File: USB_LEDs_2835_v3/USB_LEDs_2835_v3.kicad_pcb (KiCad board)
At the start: 2 copper layers, 159 x 133.3 mm, 389 parts, among them J12 Screw_Terminal_01x03, J13 Barrel_Jack_Switch, U1 MT9284, U16 MT9284, U17 JL8022W-L, U18 74LVC1G04, U19 MT9284, U2 JL8022W-L, U20 JL8022W-L, U21 74LVC1G04, U22 MT9284, U23 JL8022W-L, U24 74LVC1G04, U25 MT9284, U26 JL8022W-L, U27 74LVC1G04, U3 74LVC1G04

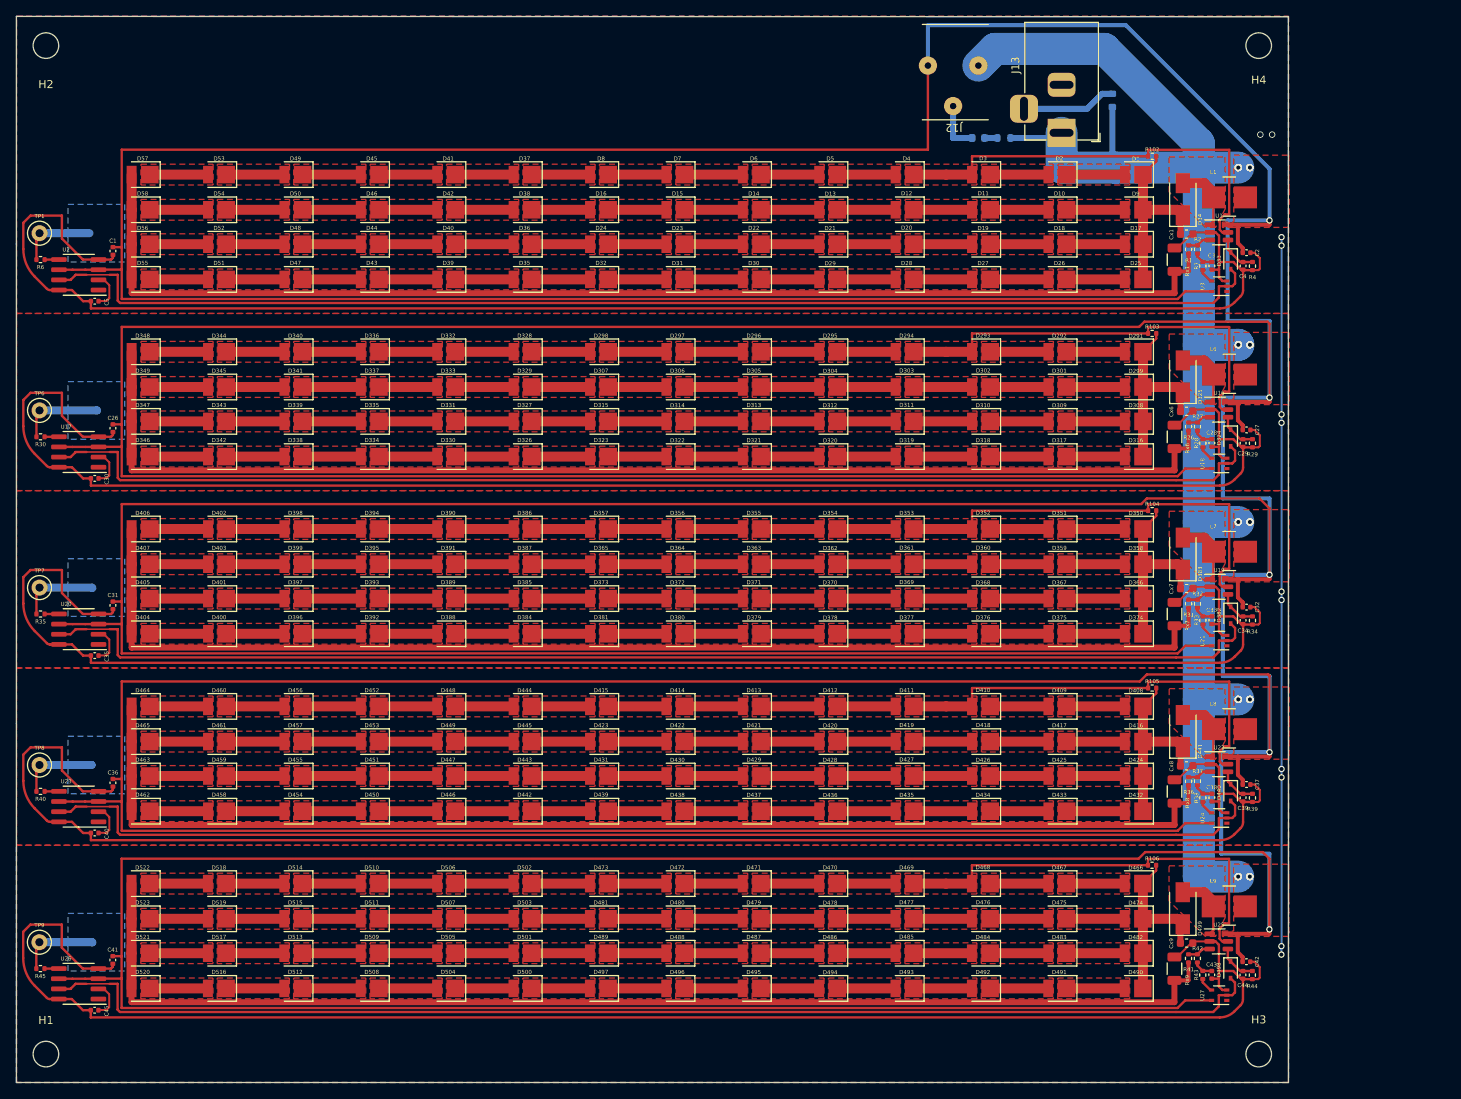
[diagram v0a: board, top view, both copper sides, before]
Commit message: Add files via upload
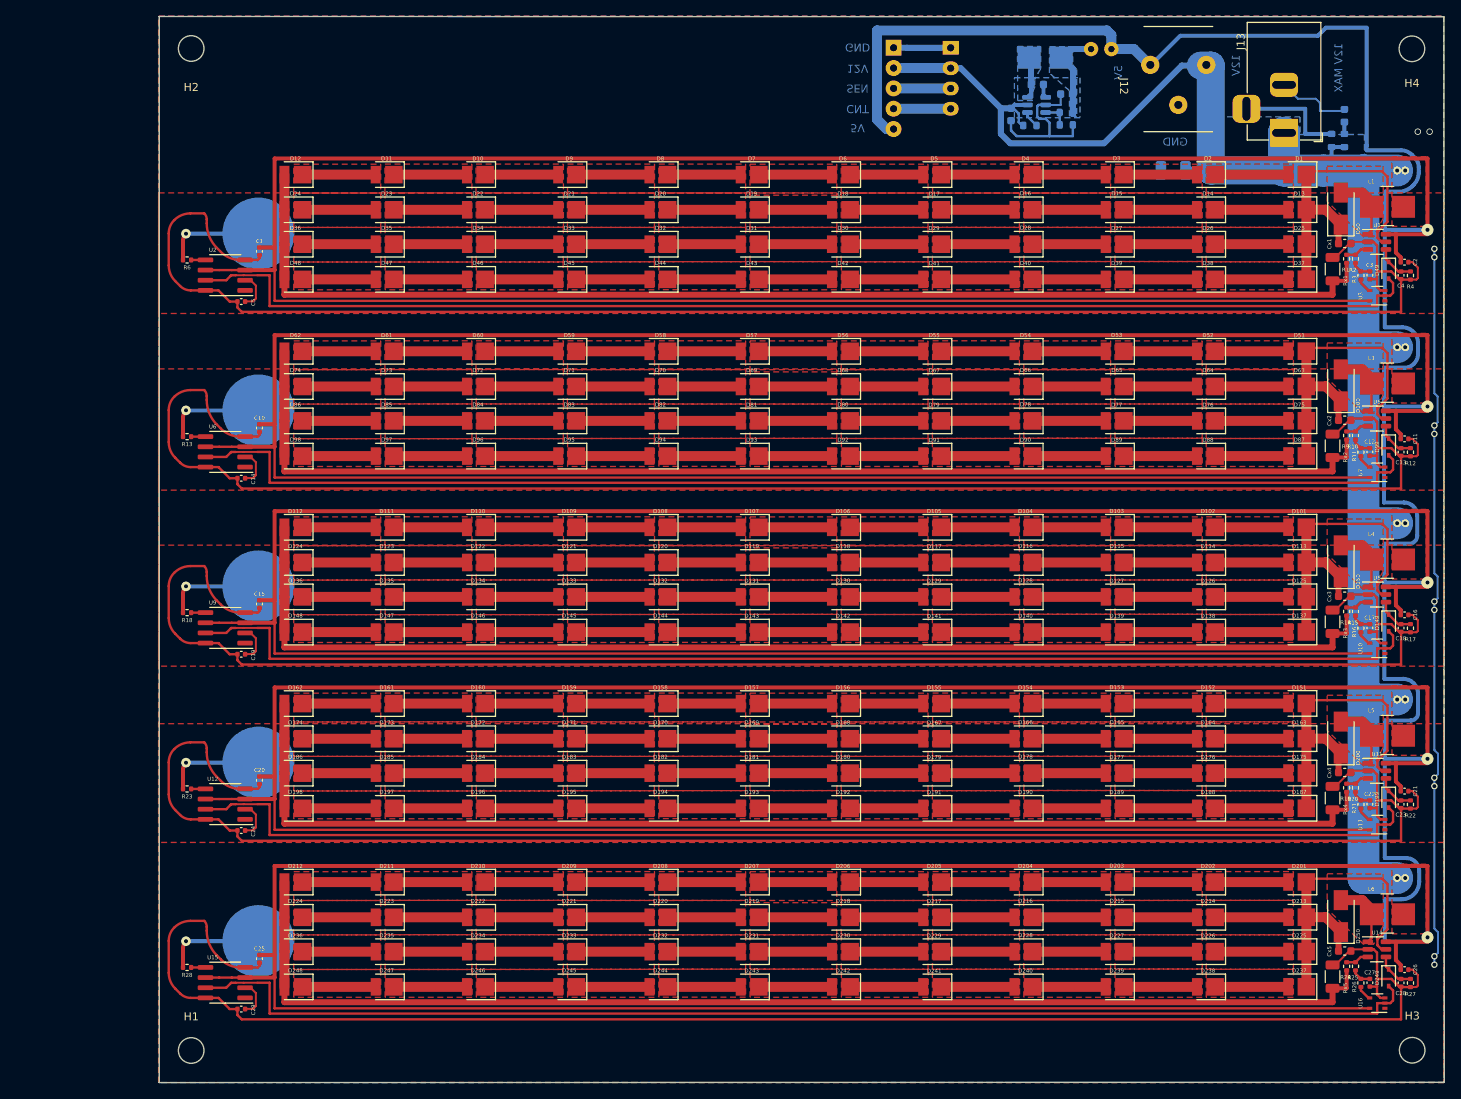
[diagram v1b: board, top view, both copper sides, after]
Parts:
- removed C30, C35, C40, C45: 10n, Capacitor_SMD:C_0402_1005Metric
- removed C31, C32, C33, C36, C37, C38, C41, C42, C43: 1u, Capacitor_SMD:C_0402_1005Metric
- removed C34, C39, C44: 1n, Capacitor_SMD:C_0402_1005Metric
- removed Cx6, Cx7, Cx8, Cx9: 1u, Capacitor_SMD:C_0603_1608Metric
- removed D291, D292, D293, D294, D295, D296, D297, D298, D299, D301, D302, D303, D304, D305, D306, D307, D308, D309, D310, D311, D312, D313, D314, D315, D316, D317, D318, D319, D320, D321, D322, D323, D326, D327, D328, D329, D330, D331, D332, D333, D334, D335, D336, D337, D338, D339, D340, D341, D342, D343, D344, D345, D346, D347, D348, D349, D350, D351, D352, D353, D354, D355, D356, D357, D358, D359, D360, D361, D362, D363, D364, D365, D366, D367, D368, D369, D370, D371, D372, D373, D374, D375, D376, D377, D378, D379, D380, D381, D384, D385, D386, D387, D388, D389, D390, D391, D392, D393, D394, D395, D396, D397, D398, D399, D400, D401, D402, D403, D404, D405, D406, D407, D408, D409, D410, D411, D412, D413, D414, D415, D416, D417, D418, D419, D420, D421, D422, D423, D424, D425, D426, D427, D428, D429, D430, D431, D432, D433, D434, D435, D436, D437, D438, D439, D442, D443, D444, D445, D446, D447, D448, D449, D450, D451, D452, D453, D454, D455, D456, D457, D458, D459, D460, D461, D462, D463, D464, D465, D466, D467, D468, D469, D470, D471, D472, D473, D474, D475, D476, D477, D478, D479, D480, D481, D482, D483, D484, D485, D486, D487, D488, D489, D490, D491, D492, D493, D494, D495, D496, D497, D500, D501, D502, D503, D504, D505, D506, D507, D508, D509, D510, D511, D512, D513, D514, D515, D516, D517, D518, D519, D520, D521, D522, D523: 660nm, LED_SMD:LED_2835
- removed D324, D382, D440, D498: 1N4148WS, Diode_SMD:D_SOD-323
- removed D325, D383, D441, D499: SS14, Diode_SMD:D_SMA
- removed L7, L8, L9: L_Ferrite_Small, Inductor_SMD:L_0530_custom
- removed R102, R103, R104, R105, R106: 500k, Resistor_SMD:R_0402_1005Metric
- removed R29, R34, R39, R44: 100k, Resistor_SMD:R_0402_1005Metric
- removed R30, R31, R35, R36, R40, R41, R45: 5k, Resistor_SMD:R_0402_1005Metric
- removed R32, R33, R37, R38, R42, R43: 10k, Resistor_SMD:R_0402_1005Metric
- removed Rx6, Rx7, Rx8, Rx9: 100m, Resistor_SMD:R_1206_3216Metric
- removed TP1, TP6, TP7, TP8, TP9: TestPoint, TestPoint:TestPoint_Loop_D2.50mm_Drill1.0mm
- removed U17, U20, U23, U26: JL8022W-L, Package_SO:SOIC-8_3.9x4.9mm_P1.27mm
- removed U18, U21, U24, U27: 74LVC1G04, Package_TO_SOT_SMD:SOT-353_SC-70-5
- removed U19, U22, U25: MT9284, Package_TO_SOT_SMD:SOT-23-6
- added ?: , , F.Cu at (82.5, 139.3)
- added ?: , , F.Cu at (82.5, 95.0)
- added ?: , , F.Cu at (82.5, 73.0)
- added ?: , , F.Cu at (82.5, 117.0)
- added C10: 1u, Capacitor_SMD:C_0402_1005Metric, F.Cu at (82.6, 75.2)
- added C11: 1u, Capacitor_SMD:C_0402_1005Metric, F.Cu at (225.7, 76.5)
- added C12: 1u, Capacitor_SMD:C_0402_1005Metric, F.Cu at (221.4, 78.2)
- added C13: 1n, Capacitor_SMD:C_0402_1005Metric, F.Cu at (225.3, 78.2)
- added C14: 10n, Capacitor_SMD:C_0402_1005Metric, F.Cu at (80.3, 81.5)
- added C15: 1u, Capacitor_SMD:C_0402_1005Metric, F.Cu at (82.6, 97.2)
- added C16: 1u, Capacitor_SMD:C_0402_1005Metric, F.Cu at (225.7, 98.5)
- added C17: 1u, Capacitor_SMD:C_0402_1005Metric, F.Cu at (221.4, 100.2)
- added C18: 1n, Capacitor_SMD:C_0402_1005Metric, F.Cu at (225.3, 100.2)
- added C19: 10n, Capacitor_SMD:C_0402_1005Metric, F.Cu at (80.3, 103.5)
- added C20: 1u, Capacitor_SMD:C_0402_1005Metric, F.Cu at (82.6, 119.2)
- added C21: 1u, Capacitor_SMD:C_0402_1005Metric, F.Cu at (225.7, 120.6)
- added C22: 1u, Capacitor_SMD:C_0402_1005Metric, F.Cu at (221.4, 122.2)
- added C23: 1n, Capacitor_SMD:C_0402_1005Metric, F.Cu at (225.3, 122.2)
- added C24: 10n, Capacitor_SMD:C_0402_1005Metric, F.Cu at (80.3, 125.5)
- added C25: 1u, Capacitor_SMD:C_0402_1005Metric, F.Cu at (82.6, 141.5)
- added C6: 22u, Capacitor_SMD:C_0603_1608Metric, B.Cu at (176.5, 36.0)
- added C7: 200n, Capacitor_SMD:C_0603_1608Metric, B.Cu at (179.8, 32.2)
- added C8: 22u, Capacitor_SMD:C_0603_1608Metric, B.Cu at (183.5, 33.5)
- added C9: 100u/16V, Capacitor_Tantalum_SMD:CP_EIA-3528-21_Kemet-B, B.Cu at (196.8, 43.0)
- added Cx2: 1u, Capacitor_SMD:C_0603_1608Metric, F.Cu at (218.2, 74.2)
- added Cx3: 1u, Capacitor_SMD:C_0603_1608Metric, F.Cu at (218.2, 96.2)
- added Cx4: 1u, Capacitor_SMD:C_0603_1608Metric, F.Cu at (218.2, 118.2)
- added Cx5: 1u, Capacitor_SMD:C_0603_1608Metric, F.Cu at (218.2, 140.6)
- added D100: SS14, Diode_SMD:D_SMA, F.Cu at (217.8, 69.9)
- added D101: 660nm, LED_SMD:LED_2835, F.Cu at (212.6, 87.6)
- added D102: 660nm, LED_SMD:LED_2835, F.Cu at (201.1, 87.6)
- added D103: 660nm, LED_SMD:LED_2835, F.Cu at (189.7, 87.6)
- added D104: 660nm, LED_SMD:LED_2835, F.Cu at (178.3, 87.6)
- added D105: 660nm, LED_SMD:LED_2835, F.Cu at (166.9, 87.6)
- added D106: 660nm, LED_SMD:LED_2835, F.Cu at (155.5, 87.6)
- added D107: 660nm, LED_SMD:LED_2835, F.Cu at (144.1, 87.6)
- added D108: 660nm, LED_SMD:LED_2835, F.Cu at (132.7, 87.6)
- added D109: 660nm, LED_SMD:LED_2835, F.Cu at (121.3, 87.6)
- added D110: 660nm, LED_SMD:LED_2835, F.Cu at (109.9, 87.6)
- added D111: 660nm, LED_SMD:LED_2835, F.Cu at (98.5, 87.6)
- added D112: 660nm, LED_SMD:LED_2835, F.Cu at (87.1, 87.6)
- added D113: 660nm, LED_SMD:LED_2835, F.Cu at (212.6, 92.0)
- added D114: 660nm, LED_SMD:LED_2835, F.Cu at (201.1, 92.0)
- added D115: 660nm, LED_SMD:LED_2835, F.Cu at (189.7, 92.0)
- added D116: 660nm, LED_SMD:LED_2835, F.Cu at (178.3, 92.0)
- added D117: 660nm, LED_SMD:LED_2835, F.Cu at (166.9, 92.0)
- added D118: 660nm, LED_SMD:LED_2835, F.Cu at (155.5, 92.0)
- added D119: 660nm, LED_SMD:LED_2835, F.Cu at (144.1, 92.0)
- added D120: 660nm, LED_SMD:LED_2835, F.Cu at (132.7, 92.0)
- added D121: 660nm, LED_SMD:LED_2835, F.Cu at (121.3, 92.0)
- added D122: 660nm, LED_SMD:LED_2835, F.Cu at (109.9, 92.0)
- added D123: 660nm, LED_SMD:LED_2835, F.Cu at (98.5, 92.0)
- added D124: 660nm, LED_SMD:LED_2835, F.Cu at (87.1, 92.0)
- added D125: 660nm, LED_SMD:LED_2835, F.Cu at (212.6, 96.3)
- added D126: 660nm, LED_SMD:LED_2835, F.Cu at (201.1, 96.3)
- added D127: 660nm, LED_SMD:LED_2835, F.Cu at (189.7, 96.3)
- added D128: 660nm, LED_SMD:LED_2835, F.Cu at (178.3, 96.3)
- added D129: 660nm, LED_SMD:LED_2835, F.Cu at (166.9, 96.3)
- added D130: 660nm, LED_SMD:LED_2835, F.Cu at (155.5, 96.3)
- added D131: 660nm, LED_SMD:LED_2835, F.Cu at (144.1, 96.3)
- added D132: 660nm, LED_SMD:LED_2835, F.Cu at (132.7, 96.3)
- added D133: 660nm, LED_SMD:LED_2835, F.Cu at (121.3, 96.3)
- added D134: 660nm, LED_SMD:LED_2835, F.Cu at (109.9, 96.3)
- added D135: 660nm, LED_SMD:LED_2835, F.Cu at (98.5, 96.3)
- added D136: 660nm, LED_SMD:LED_2835, F.Cu at (87.1, 96.3)
- added D137: 660nm, LED_SMD:LED_2835, F.Cu at (212.6, 100.7)
- added D138: 660nm, LED_SMD:LED_2835, F.Cu at (201.1, 100.7)
- added D139: 660nm, LED_SMD:LED_2835, F.Cu at (189.7, 100.7)
- added D140: 660nm, LED_SMD:LED_2835, F.Cu at (178.3, 100.7)
- added D141: 660nm, LED_SMD:LED_2835, F.Cu at (166.9, 100.7)
- added D142: 660nm, LED_SMD:LED_2835, F.Cu at (155.5, 100.7)
- added D143: 660nm, LED_SMD:LED_2835, F.Cu at (144.1, 100.7)
- added D144: 660nm, LED_SMD:LED_2835, F.Cu at (132.7, 100.7)
- added D145: 660nm, LED_SMD:LED_2835, F.Cu at (121.3, 100.7)
- added D146: 660nm, LED_SMD:LED_2835, F.Cu at (109.9, 100.7)
- added D147: 660nm, LED_SMD:LED_2835, F.Cu at (98.5, 100.7)
- added D148: 660nm, LED_SMD:LED_2835, F.Cu at (87.1, 100.7)
- added D149: 1N4148WS, Diode_SMD:D_SOD-323, F.Cu at (223.7, 99.6)
- added D150: SS14, Diode_SMD:D_SMA, F.Cu at (217.8, 91.9)
- added D151: 660nm, LED_SMD:LED_2835, F.Cu at (212.6, 109.6)
- added D152: 660nm, LED_SMD:LED_2835, F.Cu at (201.1, 109.6)
- added D153: 660nm, LED_SMD:LED_2835, F.Cu at (189.7, 109.6)
- added D154: 660nm, LED_SMD:LED_2835, F.Cu at (178.3, 109.6)
- added D155: 660nm, LED_SMD:LED_2835, F.Cu at (166.9, 109.6)
- added D156: 660nm, LED_SMD:LED_2835, F.Cu at (155.5, 109.6)
- added D157: 660nm, LED_SMD:LED_2835, F.Cu at (144.1, 109.6)
- added D158: 660nm, LED_SMD:LED_2835, F.Cu at (132.7, 109.6)
- added D159: 660nm, LED_SMD:LED_2835, F.Cu at (121.3, 109.6)
- added D160: 660nm, LED_SMD:LED_2835, F.Cu at (109.9, 109.6)
- added D161: 660nm, LED_SMD:LED_2835, F.Cu at (98.5, 109.6)
- added D162: 660nm, LED_SMD:LED_2835, F.Cu at (87.1, 109.6)
- added D163: 660nm, LED_SMD:LED_2835, F.Cu at (212.6, 114.0)
- added D164: 660nm, LED_SMD:LED_2835, F.Cu at (201.1, 114.0)
- added D165: 660nm, LED_SMD:LED_2835, F.Cu at (189.7, 114.0)
- added D166: 660nm, LED_SMD:LED_2835, F.Cu at (178.3, 114.0)
- added D167: 660nm, LED_SMD:LED_2835, F.Cu at (166.9, 114.0)
- added D168: 660nm, LED_SMD:LED_2835, F.Cu at (155.5, 114.0)
- added D169: 660nm, LED_SMD:LED_2835, F.Cu at (144.1, 114.0)
- added D170: 660nm, LED_SMD:LED_2835, F.Cu at (132.7, 114.0)
- added D171: 660nm, LED_SMD:LED_2835, F.Cu at (121.3, 114.0)
- added D172: 660nm, LED_SMD:LED_2835, F.Cu at (109.9, 114.0)
- added D173: 660nm, LED_SMD:LED_2835, F.Cu at (98.5, 114.0)
- added D174: 660nm, LED_SMD:LED_2835, F.Cu at (87.1, 114.0)
- added D175: 660nm, LED_SMD:LED_2835, F.Cu at (212.6, 118.3)
- added D176: 660nm, LED_SMD:LED_2835, F.Cu at (201.1, 118.3)
- added D177: 660nm, LED_SMD:LED_2835, F.Cu at (189.7, 118.3)
- added D178: 660nm, LED_SMD:LED_2835, F.Cu at (178.3, 118.3)
- added D179: 660nm, LED_SMD:LED_2835, F.Cu at (166.9, 118.3)
- added D180: 660nm, LED_SMD:LED_2835, F.Cu at (155.5, 118.3)
- added D181: 660nm, LED_SMD:LED_2835, F.Cu at (144.1, 118.3)
- added D182: 660nm, LED_SMD:LED_2835, F.Cu at (132.7, 118.3)
- added D183: 660nm, LED_SMD:LED_2835, F.Cu at (121.3, 118.3)
- added D184: 660nm, LED_SMD:LED_2835, F.Cu at (109.9, 118.3)
- added D185: 660nm, LED_SMD:LED_2835, F.Cu at (98.5, 118.3)
- added D186: 660nm, LED_SMD:LED_2835, F.Cu at (87.1, 118.3)
- added D187: 660nm, LED_SMD:LED_2835, F.Cu at (212.6, 122.7)
- added D188: 660nm, LED_SMD:LED_2835, F.Cu at (201.1, 122.7)
- added D189: 660nm, LED_SMD:LED_2835, F.Cu at (189.7, 122.7)
- added D190: 660nm, LED_SMD:LED_2835, F.Cu at (178.3, 122.7)
- added D191: 660nm, LED_SMD:LED_2835, F.Cu at (166.9, 122.7)
- added D192: 660nm, LED_SMD:LED_2835, F.Cu at (155.5, 122.7)
- added D193: 660nm, LED_SMD:LED_2835, F.Cu at (144.1, 122.7)
- added D194: 660nm, LED_SMD:LED_2835, F.Cu at (132.7, 122.7)
- added D195: 660nm, LED_SMD:LED_2835, F.Cu at (121.3, 122.7)
- added D196: 660nm, LED_SMD:LED_2835, F.Cu at (109.9, 122.7)
- added D197: 660nm, LED_SMD:LED_2835, F.Cu at (98.5, 122.7)
- added D198: 660nm, LED_SMD:LED_2835, F.Cu at (87.1, 122.7)
- added D199: 1N4148WS, Diode_SMD:D_SOD-323, F.Cu at (223.7, 121.6)
- added D200: SS14, Diode_SMD:D_SMA, F.Cu at (217.8, 113.9)
- added D201: 660nm, LED_SMD:LED_2835, F.Cu at (212.6, 131.9)
- added D202: 660nm, LED_SMD:LED_2835, F.Cu at (201.1, 131.9)
- added D203: 660nm, LED_SMD:LED_2835, F.Cu at (189.7, 131.9)
- added D204: 660nm, LED_SMD:LED_2835, F.Cu at (178.3, 131.9)
- added D205: 660nm, LED_SMD:LED_2835, F.Cu at (166.9, 131.9)
- added D206: 660nm, LED_SMD:LED_2835, F.Cu at (155.5, 131.9)
- added D207: 660nm, LED_SMD:LED_2835, F.Cu at (144.1, 131.9)
- added D208: 660nm, LED_SMD:LED_2835, F.Cu at (132.7, 131.9)
- added D209: 660nm, LED_SMD:LED_2835, F.Cu at (121.3, 131.9)
- added D210: 660nm, LED_SMD:LED_2835, F.Cu at (109.9, 131.9)
- added D211: 660nm, LED_SMD:LED_2835, F.Cu at (98.5, 131.9)
- added D212: 660nm, LED_SMD:LED_2835, F.Cu at (87.1, 131.9)
- added D213: 660nm, LED_SMD:LED_2835, F.Cu at (212.6, 136.3)
- added D214: 660nm, LED_SMD:LED_2835, F.Cu at (201.1, 136.3)
- added D215: 660nm, LED_SMD:LED_2835, F.Cu at (189.7, 136.3)
- added D216: 660nm, LED_SMD:LED_2835, F.Cu at (178.3, 136.3)
- added D217: 660nm, LED_SMD:LED_2835, F.Cu at (166.9, 136.3)
- added D218: 660nm, LED_SMD:LED_2835, F.Cu at (155.5, 136.3)
- added D219: 660nm, LED_SMD:LED_2835, F.Cu at (144.1, 136.3)
- added D220: 660nm, LED_SMD:LED_2835, F.Cu at (132.7, 136.3)
- added D221: 660nm, LED_SMD:LED_2835, F.Cu at (121.3, 136.3)
- added D222: 660nm, LED_SMD:LED_2835, F.Cu at (109.9, 136.3)
- added D223: 660nm, LED_SMD:LED_2835, F.Cu at (98.5, 136.3)
- added D224: 660nm, LED_SMD:LED_2835, F.Cu at (87.1, 136.3)
- added D225: 660nm, LED_SMD:LED_2835, F.Cu at (212.6, 140.6)
- added D226: 660nm, LED_SMD:LED_2835, F.Cu at (201.1, 140.7)
- added D227: 660nm, LED_SMD:LED_2835, F.Cu at (189.7, 140.7)
- added D228: 660nm, LED_SMD:LED_2835, F.Cu at (178.3, 140.7)
- added D229: 660nm, LED_SMD:LED_2835, F.Cu at (166.9, 140.7)
- added D230: 660nm, LED_SMD:LED_2835, F.Cu at (155.5, 140.7)
- added D231: 660nm, LED_SMD:LED_2835, F.Cu at (144.1, 140.7)
- added D232: 660nm, LED_SMD:LED_2835, F.Cu at (132.7, 140.7)
- added D233: 660nm, LED_SMD:LED_2835, F.Cu at (121.3, 140.7)
- added D234: 660nm, LED_SMD:LED_2835, F.Cu at (109.9, 140.7)
- added D235: 660nm, LED_SMD:LED_2835, F.Cu at (98.5, 140.7)
- added D236: 660nm, LED_SMD:LED_2835, F.Cu at (87.1, 140.7)
- added D237: 660nm, LED_SMD:LED_2835, F.Cu at (212.6, 145.0)
- added D238: 660nm, LED_SMD:LED_2835, F.Cu at (201.1, 145.1)
- added D239: 660nm, LED_SMD:LED_2835, F.Cu at (189.7, 145.1)
- added D240: 660nm, LED_SMD:LED_2835, F.Cu at (178.3, 145.1)
- added D241: 660nm, LED_SMD:LED_2835, F.Cu at (166.9, 145.1)
- added D242: 660nm, LED_SMD:LED_2835, F.Cu at (155.5, 145.1)
- added D243: 660nm, LED_SMD:LED_2835, F.Cu at (144.1, 145.1)
- added D244: 660nm, LED_SMD:LED_2835, F.Cu at (132.7, 145.1)
- added D245: 660nm, LED_SMD:LED_2835, F.Cu at (121.3, 145.1)
- added D246: 660nm, LED_SMD:LED_2835, F.Cu at (109.9, 145.1)
- added D247: 660nm, LED_SMD:LED_2835, F.Cu at (98.5, 145.1)
- added D248: 660nm, LED_SMD:LED_2835, F.Cu at (87.1, 145.1)
- added D249: 1N4148WS, Diode_SMD:D_SOD-323, F.Cu at (223.7, 143.9)
- added D250: SS14, Diode_SMD:D_SMA, F.Cu at (217.8, 136.2)
- added D59: 660nm, LED_SMD:LED_2835, F.Cu at (121.3, 65.6)
- added D60: 660nm, LED_SMD:LED_2835, F.Cu at (109.9, 65.6)
- added D61: 660nm, LED_SMD:LED_2835, F.Cu at (98.5, 65.6)
- added D62: 660nm, LED_SMD:LED_2835, F.Cu at (87.1, 65.6)
- added D63: 660nm, LED_SMD:LED_2835, F.Cu at (212.6, 70.0)
- added D64: 660nm, LED_SMD:LED_2835, F.Cu at (201.1, 70.0)
- added D65: 660nm, LED_SMD:LED_2835, F.Cu at (189.7, 70.0)
- added D66: 660nm, LED_SMD:LED_2835, F.Cu at (178.3, 70.0)
- added D67: 660nm, LED_SMD:LED_2835, F.Cu at (166.9, 70.0)
- added D68: 660nm, LED_SMD:LED_2835, F.Cu at (155.5, 70.0)
- added D69: 660nm, LED_SMD:LED_2835, F.Cu at (144.1, 70.0)
- added D70: 660nm, LED_SMD:LED_2835, F.Cu at (132.7, 70.0)
- added D71: 660nm, LED_SMD:LED_2835, F.Cu at (121.3, 70.0)
- added D72: 660nm, LED_SMD:LED_2835, F.Cu at (109.9, 70.0)
- added D73: 660nm, LED_SMD:LED_2835, F.Cu at (98.5, 70.0)
- added D74: 660nm, LED_SMD:LED_2835, F.Cu at (87.1, 70.0)
- added D75: 660nm, LED_SMD:LED_2835, F.Cu at (212.6, 74.3)
- added D76: 660nm, LED_SMD:LED_2835, F.Cu at (201.1, 74.3)
- added D77: 660nm, LED_SMD:LED_2835, F.Cu at (189.7, 74.3)
- added D78: 660nm, LED_SMD:LED_2835, F.Cu at (178.3, 74.3)
- added D79: 660nm, LED_SMD:LED_2835, F.Cu at (166.9, 74.3)
- added D80: 660nm, LED_SMD:LED_2835, F.Cu at (155.5, 74.3)
- added D81: 660nm, LED_SMD:LED_2835, F.Cu at (144.1, 74.3)
- added D82: 660nm, LED_SMD:LED_2835, F.Cu at (132.7, 74.3)
- added D83: 660nm, LED_SMD:LED_2835, F.Cu at (121.3, 74.3)
- added D84: 660nm, LED_SMD:LED_2835, F.Cu at (109.9, 74.3)
- added D85: 660nm, LED_SMD:LED_2835, F.Cu at (98.5, 74.3)
- added D86: 660nm, LED_SMD:LED_2835, F.Cu at (87.1, 74.3)
- added D87: 660nm, LED_SMD:LED_2835, F.Cu at (212.6, 78.7)
- added D88: 660nm, LED_SMD:LED_2835, F.Cu at (201.1, 78.7)
- added D89: 660nm, LED_SMD:LED_2835, F.Cu at (189.7, 78.7)
- added D90: 660nm, LED_SMD:LED_2835, F.Cu at (178.3, 78.7)
- added D91: 660nm, LED_SMD:LED_2835, F.Cu at (166.9, 78.7)
- added D92: 660nm, LED_SMD:LED_2835, F.Cu at (155.5, 78.7)
- added D93: 660nm, LED_SMD:LED_2835, F.Cu at (144.1, 78.7)
- added D94: 660nm, LED_SMD:LED_2835, F.Cu at (132.7, 78.7)
- added D95: 660nm, LED_SMD:LED_2835, F.Cu at (121.3, 78.7)
- added D96: 660nm, LED_SMD:LED_2835, F.Cu at (109.9, 78.7)
- added D97: 660nm, LED_SMD:LED_2835, F.Cu at (98.5, 78.7)
- added D98: 660nm, LED_SMD:LED_2835, F.Cu at (87.1, 78.7)
- added D99: 1N4148WS, Diode_SMD:D_SOD-323, F.Cu at (223.7, 77.6)
- added J1: external header, Connector_PinHeader_2.54mm:PinHeader_1x05_P2.54mm_Vertical, B.Cu at (161.8, 27.7)
- added J2: Fan conn, Connector:FanPinHeader_1x04_P2.54mm_Vertical_custom, B.Cu at (169.0, 27.7)
- added JP1: j_open, TestPoint:TestPoint_2Pads_Pitch2.54mm_Drill0.8mm, B.Cu at (186.5, 27.8)
- added L2: 4.7u, Inductor_SMD:L_0530_custom, B.Cu at (180.8, 28.9)
- added L3: L_Ferrite_Small, Inductor_SMD:L_0530_custom, F.Cu at (223.6, 69.6)
- added L4: L_Ferrite_Small, Inductor_SMD:L_0530_custom, F.Cu at (223.6, 91.6)
- added L5: L_Ferrite_Small, Inductor_SMD:L_0530_custom, F.Cu at (223.6, 113.7)
- added R10: 10k, Resistor_SMD:R_0402_1005Metric, F.Cu at (219.6, 76.1)
- added R11: 10k, Resistor_SMD:R_0402_1005Metric, F.Cu at (220.3, 78.2)
- added R12: 100k, Resistor_SMD:R_0402_1005Metric, F.Cu at (226.5, 78.2)
- added R13: 5k, Resistor_SMD:R_0402_1005Metric, F.Cu at (73.5, 76.3)
- added R14: 5k, Resistor_SMD:R_0402_1005Metric, F.Cu at (218.5, 98.1)
- added R15: 10k, Resistor_SMD:R_0402_1005Metric, F.Cu at (219.6, 98.1)
- added R16: 10k, Resistor_SMD:R_0402_1005Metric, F.Cu at (220.3, 100.2)
- added R17: 100k, Resistor_SMD:R_0402_1005Metric, F.Cu at (226.5, 100.2)
- added R18: 5k, Resistor_SMD:R_0402_1005Metric, F.Cu at (73.5, 98.3)
- added R19: 5k, Resistor_SMD:R_0402_1005Metric, F.Cu at (218.5, 120.2)
- added R20: 10k, Resistor_SMD:R_0402_1005Metric, F.Cu at (219.6, 120.2)
- added R21: 10k, Resistor_SMD:R_0402_1005Metric, F.Cu at (220.3, 122.2)
- added R22: 100k, Resistor_SMD:R_0402_1005Metric, F.Cu at (226.5, 122.2)
- added R23: 5k, Resistor_SMD:R_0402_1005Metric, F.Cu at (73.5, 120.3)
- added R24: 5k, Resistor_SMD:R_0402_1005Metric, F.Cu at (218.5, 142.5)
- added R25: 10k, Resistor_SMD:R_0402_1005Metric, F.Cu at (219.6, 142.5)
- added R5: 51k, Resistor_SMD:R_0603_1608Metric, B.Cu at (183.4, 35.8)
- added R7: 6.8k, Resistor_SMD:R_0603_1608Metric, B.Cu at (183.4, 37.3)
- added R8: 22k, Resistor_SMD:R_0603_1608Metric, B.Cu at (178.9, 37.4)
- added R9: 5k, Resistor_SMD:R_0402_1005Metric, F.Cu at (218.5, 76.1)
- added REF**: TestPoint_Pad_D4.0mm, TestPoint:TestPoint_Pad_D4.0mm, B.Cu at (82.5, 50.9)
- added Rx2: 100m, Resistor_SMD:R_1206_3216Metric, F.Cu at (216.7, 77.4)
- added Rx3: 100m, Resistor_SMD:R_1206_3216Metric, F.Cu at (216.7, 99.4)
- added Rx4: 100m, Resistor_SMD:R_1206_3216Metric, F.Cu at (216.7, 121.5)
- added Rx5: 100m, Resistor_SMD:R_1206_3216Metric, F.Cu at (216.7, 143.8)
- added U10: 74LVC1G04, Package_TO_SOT_SMD:SOT-353_SC-70-5, F.Cu at (222.3, 102.7)
- added U11: MT9284, Package_TO_SOT_SMD:SOT-23-6, F.Cu at (222.3, 118.0)
- added U12: JL8022W-L, Package_SO:SOIC-8_3.9x4.9mm_P1.27mm, F.Cu at (78.3, 122.2)
- added U13: 74LVC1G04, Package_TO_SOT_SMD:SOT-353_SC-70-5, F.Cu at (222.3, 124.8)
- added U14: MT9284, Package_TO_SOT_SMD:SOT-23-6, F.Cu at (222.3, 140.4)
- added U15: JL8022W-L, Package_SO:SOIC-8_3.9x4.9mm_P1.27mm, F.Cu at (78.3, 144.5)
- added U4: STI3470, Package_TO_SOT_SMD:SOT-23-6, B.Cu at (179.7, 34.8)
- added U5: MT9284, Package_TO_SOT_SMD:SOT-23-6, F.Cu at (222.3, 74.0)
- added U6: JL8022W-L, Package_SO:SOIC-8_3.9x4.9mm_P1.27mm, F.Cu at (78.3, 78.2)
- added U7: 74LVC1G04, Package_TO_SOT_SMD:SOT-353_SC-70-5, F.Cu at (222.3, 80.7)
- added U8: MT9284, Package_TO_SOT_SMD:SOT-23-6, F.Cu at (222.3, 96.0)
- added U9: JL8022W-L, Package_SO:SOIC-8_3.9x4.9mm_P1.27mm, F.Cu at (78.3, 100.2)
- C28: value 1u -> 1n
- C29: value 1n -> 10n
- R26: value 5k -> 10k
- R27: value 10k -> 100k
- R28: value 10k -> 5k
- U16: value MT9284 -> 74LVC1G04; footprint Package_TO_SOT_SMD:SOT-23-6 -> Package_TO_SOT_SMD:SOT-353_SC-70-5
- moved C26 175.1 mm to (225.7, 142.9), turned to 0 degrees
- moved C29 143.8 mm to (80.3, 147.8), turned to 180 degrees
- moved R28 142.9 mm to (73.5, 142.6), turned to 0 degrees
- moved D51 135.3 mm to (212.6, 65.6)
- moved D52 124.3 mm to (201.1, 65.6)
- moved D53 114.4 mm to (189.7, 65.6)
- moved D54 102.3 mm to (178.3, 65.6)
- moved D55 99.4 mm to (166.9, 65.6)
- moved D56 88.6 mm to (155.5, 65.6)
- moved D57 79.3 mm to (144.1, 65.6)
- moved U16 76.8 mm to (222.3, 147.1), turned to 180 degrees
- moved R27 74.5 mm to (226.5, 144.6), turned to 90 degrees
- moved R26 72.8 mm to (220.3, 144.6)
- moved C28 71.5 mm to (225.3, 144.5)
- moved C27 70.8 mm to (221.4, 144.5), turned to -90 degrees
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- renumbered D41 to D10, D45 to D11, D49 to D12, D9 to D13, D10 to D14, D11 to D15, D12 to D16, D13 to D17, D14 to D18, D15 to D19, D16 to D20, D38 to D21, D42 to D22, D46 to D23, D50 to D24, D17 to D25, D18 to D26, D19 to D27, D20 to D28, D21 to D29, D22 to D30, D23 to D31, D24 to D32, D36 to D33, D40 to D34, D44 to D35, D48 to D36, D25 to D37, D26 to D38, D27 to D39, D28 to D40, D29 to D41, D30 to D42, D31 to D43, D32 to D44, D35 to D45, D39 to D46, D43 to D47, D47 to D48, D33 to D49, D34 to D50, D37 to D9
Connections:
- C26 pad 1: GND -> +5V
- C26 pad 2: +5V -> GND
- C27 pad 1: +5V -> Net-(C3-Pad1)
- C28 pad 1: Net-(C3-Pad1) -> Net-(C4-Pad1)
- C29 pad 1: Net-(C4-Pad1) -> Net-(C5-Pad1)
- D12 pad 1: Net-(D49-Pad1) -> Net-(D12-Pad1)
- D24 pad 1: Net-(D50-Pad1) -> Net-(D12-Pad1)
- D3 pad 1: Net-(U1-Pad5) -> Net-(D3-Pad1)
- D36 pad 1: Net-(D48-Pad1) -> Net-(D12-Pad1)
- D4 pad 2: Net-(U1-Pad5) -> Net-(D3-Pad1)
- D48 pad 1: Net-(D47-Pad1) (its old number) -> Net-(D12-Pad1)
- D49 pad 2: Net-(D33-Pad2) -> Net-(D49-Pad2)
- D50 pad 2: Net-(D34-Pad2) -> Net-(D50-Pad2)
- D51 pad 1: Net-(D51-Pad1) -> Net-(D1-Pad1)
- D51 pad 2: Net-(D47-Pad1) (its old number) -> Net-(Cx1-Pad1)
- D52 pad 1: Net-(D52-Pad1) -> Net-(D2-Pad1)
- D52 pad 2: Net-(D48-Pad1) -> Net-(D1-Pad1)
- D53 pad 1: Net-(D53-Pad1) -> Net-(D3-Pad1)
- D53 pad 2: Net-(D49-Pad1) -> Net-(D2-Pad1)
- D54 pad 1: Net-(D54-Pad1) -> Net-(D4-Pad1)
- D54 pad 2: Net-(D50-Pad1) -> Net-(D3-Pad1)
- D55 pad 1: Net-(D55-Pad1) -> Net-(D5-Pad1)
- D55 pad 2: Net-(D51-Pad1) -> Net-(D4-Pad1)
- D56 pad 1: Net-(D55-Pad1) -> Net-(D6-Pad1)
- D56 pad 2: Net-(D52-Pad1) -> Net-(D5-Pad1)
- D57 pad 1: Net-(D55-Pad1) -> Net-(D7-Pad1)
- D57 pad 2: Net-(D53-Pad1) -> Net-(D6-Pad1)
- D58 pad 1: Net-(D55-Pad1) -> Net-(D8-Pad1)
- D58 pad 2: Net-(D54-Pad1) -> Net-(D7-Pad1)
- D8 pad 1: Net-(D37-Pad2) -> Net-(D8-Pad1)
- D9 pad 2: Net-(D37-Pad2) -> Net-(D8-Pad1)
- L1 pad 2: Net-(D34-Pad2) -> Net-(D50-Pad2)
- L6 pad 2: Net-(D34-Pad2) -> Net-(D50-Pad2)
- R1 pad 1: Net-(D55-Pad1) -> Net-(D12-Pad1)
- R26 pad 1: Net-(D55-Pad1) -> Net-(R3-Pad1)
- R26 pad 2: Net-(R1-Pad2) -> Net-(C3-Pad1)
- R27 pad 1: Net-(R1-Pad2) -> GND
- R27 pad 2: Net-(C3-Pad1) -> Net-(C4-Pad1)
- R28 pad 1: Net-(R3-Pad1) -> Net-(R6-Pad1)
- R28 pad 2: Net-(C3-Pad1) -> Net-(R6-Pad2)
- Rx1 pad 2: Net-(D55-Pad1) -> Net-(D12-Pad1)
- U1 pad 1: Net-(D34-Pad2) -> Net-(D50-Pad2)
- U1 pad 5: Net-(U1-Pad5) -> Net-(Cx1-Pad1)
- U16 pad 1: Net-(D34-Pad2) -> unconnected-(U3-Pad1)
- U16 pad 2: GND -> Net-(D49-Pad2)
- U16 pad 3: Net-(R1-Pad2) -> GND
- U16 pad 4: Net-(C4-Pad1) -> Net-(R3-Pad1)
- U16 pad 5: Net-(U1-Pad5) -> +5V
- U2 pad 7: Net-(D33-Pad2) -> Net-(D49-Pad2)
- U3 pad 2: Net-(D33-Pad2) -> Net-(D49-Pad2)
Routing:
- net Net-(D49-Pad2): track 0.00 -> 780.1 mm
- net Net-(D33-Pad2): track 772.4 -> 0.00 mm
- net Net-(D55-Pad1): track 759.6 -> 0.00 mm
- net Net-(D12-Pad1): track 0.00 -> 758.8 mm
- net Net-(U1-Pad5): track 272.4 -> 0.00 mm
- net +5V: track 1788.3 -> 1897.0 mm
- net Net-(Cx1-Pad1): track 119.1 -> 203.4 mm
- net Net-(D3-Pad1): track 0.00 -> 45.7 mm
- net Net-(D8-Pad1): track 0.00 -> 45.7 mm
- net GND: track 1106.4 -> 1149.4 mm
- net Net-(D50-Pad2): track 0.00 -> 39.6 mm
- net Net-(D34-Pad2): track 39.6 -> 0.00 mm
- net Net-(D50-Pad1): track 36.4 -> 0.00 mm
- net Net-(D49-Pad1): track 36.4 -> 0.00 mm
- net Net-(D48-Pad1): track 36.4 -> 0.00 mm
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- added copper zone on B.Cu, net +12V
- added copper zone on B.Cu, net Net-(C7-Pad2)
- added copper zone on F.Cu, net Net-(D3-Pad1)
- added copper zone on F.Cu, net Net-(D50-Pad2)
- added copper zone on F.Cu, net Net-(D8-Pad1)
- added copper zone on B.Cu, net Net-(L2-Pad2)
- removed copper zone on F.Cu, net Net-(D34-Pad2)
- removed copper zone on F.Cu, net Net-(D37-Pad2)
- removed copper zone on F.Cu, net Net-(D47-Pad1) (its old number)
- removed copper zone on F.Cu, net Net-(D48-Pad1)
- removed copper zone on F.Cu, net Net-(D49-Pad1)
- removed copper zone on F.Cu, net Net-(D50-Pad1)
- removed copper zone on F.Cu, net Net-(D51-Pad1)
- removed copper zone on F.Cu, net Net-(D52-Pad1)
- removed copper zone on F.Cu, net Net-(D53-Pad1)
- removed copper zone on F.Cu, net Net-(D54-Pad1)
- removed copper zone on B.Cu, net Net-(R6-Pad1)
- removed copper zone on F.Cu, net Net-(U1-Pad5)
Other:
- board size 159 x 133.3 mm -> 160.6 x 133.3 mm
- board text added: "12V"
- board text added: "12V MAX"
- board text added: "5V"
- board text added: "CNT"
- board text added: "GND"
- board text added: "SEN"
